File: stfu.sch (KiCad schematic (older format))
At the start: 91 parts, among them K1 FTDI, K2 ISP, K3 I2C, K4 SERVO, K5 V_SEL, P1 CONN_1, P2 CONN_1, P3 HAND_HI, P4 HAND_LO, P5 HAND_HI, P6 HAND_LO, Q1 PNP, SW1 RST, SW2 RST, SW3 SW_MODE, SW4 SW_INC, SW5 SW_DEC, SW6 SW_ENT, U1 ATMEGA328-P, U2 HEF4051B, U3 ULN2803, U4 7809, U5 7805, X1 16MHz

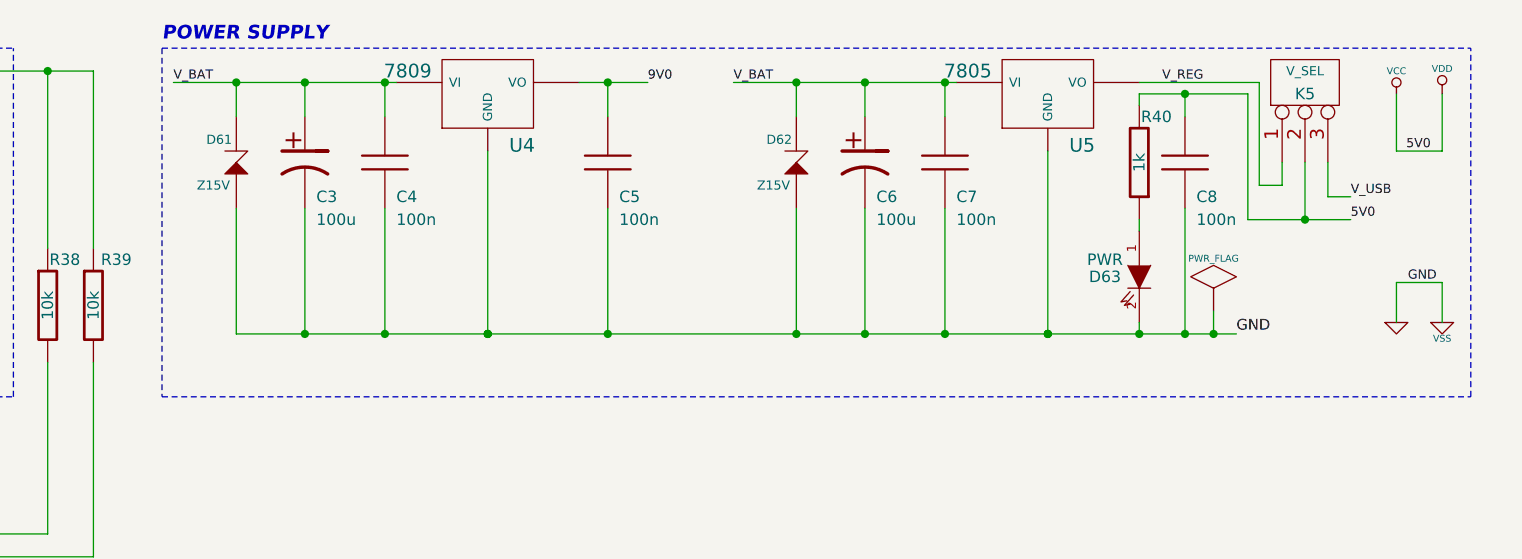
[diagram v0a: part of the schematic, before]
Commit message: preliminary board layout
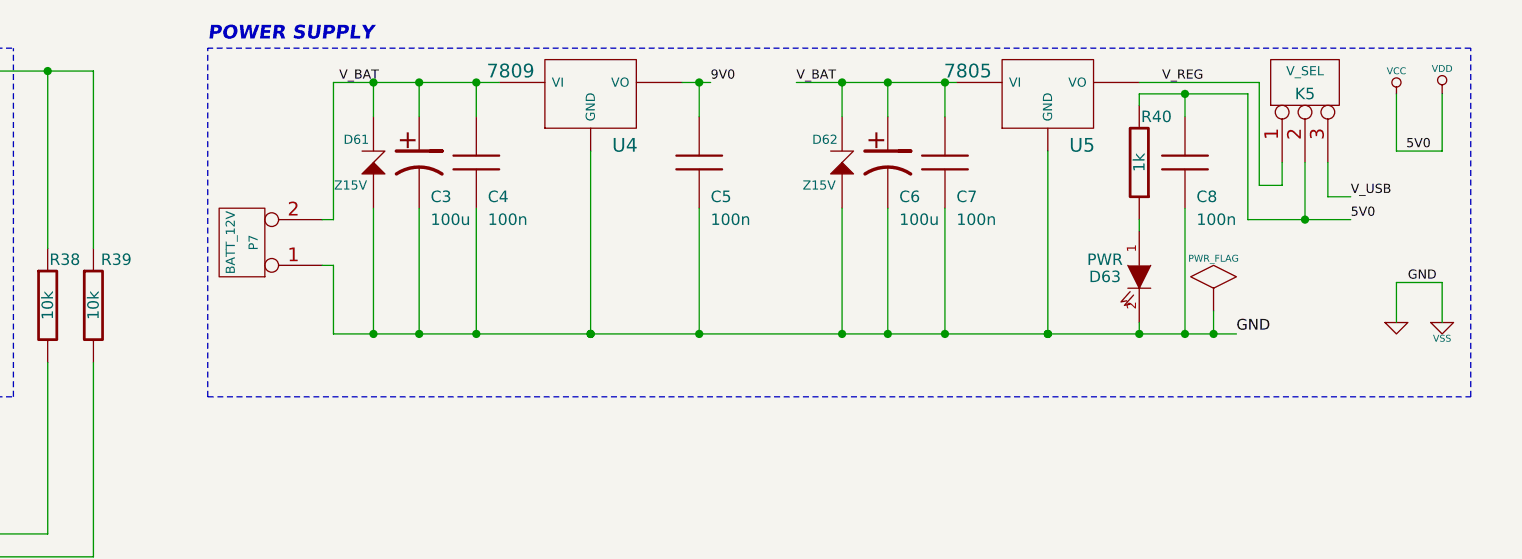
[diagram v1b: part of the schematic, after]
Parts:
- added P7: BATT_12V, symbol CONN_2
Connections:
- net GND: now also P7.1 (P1)
- net V_BAT: now also P7.2 (PM)
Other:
- moved on the sheet: C3, C4, C5, C6, D61, D62, U4
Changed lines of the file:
@@
-EESchema Schematic File Version 2  date 7/5/2012 5:41:43 PM
+EESchema Schematic File Version 2  date Monday 09 July 2012 12:59:22 AM IST
 LIBS:stfu
 LIBS:power
@@
 Sheet 1 2
 Title "STFU - a warning for incessant Noise polluters"
-Date "5 jul 2012"
+Date "8 jul 2012"
 Rev "A"
 Comp "anool.m@gmail.com"
@@
 $EndDescr
 Wire Notes Line
+	5600 2150 11125 2150
+Wire Notes Line
+	5600 2150 5600 625
+Wire Wire Line
+	6150 1375 6150 775
+Wire Wire Line
+	6150 1375 6100 1375
+Wire Notes Line
 	6950 3050 6950 4900
 Wire Notes Line
@@
 Wire Wire Line
 	6750 7325 4750 7325
-Connection ~ 8175 1875
-Wire Wire Line
-	8175 1875 8175 1325
+Connection ~ 8375 1875
+Wire Wire Line
+	8375 1875 8375 1325
 Wire Notes Line
 	3500 625  4750 625
@@
 Wire Notes Line
 	4750 2150 4750 625
-Wire Notes Line
-	5400 625  5400 2150
 Wire Wire Line
 	4900 5025 4750 5025
 Wire Wire Line
 	4750 5025 4750 5075
-Connection ~ 7350 775
-Wire Wire Line
-	7350 925  7350 775
-Connection ~ 5725 775
-Wire Wire Line
-	5725 925  5725 775
-Connection ~ 6825 1875
-Connection ~ 6375 775
-Connection ~ 6375 1875
-Wire Wire Line
-	6375 1875 6375 1325
-Connection ~ 6825 1875
-Wire Wire Line
-	6025 1325 6025 1875
-Wire Wire Line
-	6025 775  6025 925
-Wire Wire Line
-	6825 1875 6825 1075
-Wire Wire Line
-	6375 775  6375 925
-Connection ~ 6025 775
-Wire Wire Line
-	6425 775  5450 775
-Wire Wire Line
-	5725 1325 5725 1875
-Connection ~ 6025 1875
+Connection ~ 7750 775
+Wire Wire Line
+	7750 925  7750 775
+Connection ~ 6325 775
+Wire Wire Line
+	6325 775  6325 925
+Connection ~ 7275 1875
+Connection ~ 6775 775
+Connection ~ 6775 1875
+Wire Wire Line
+	6775 1875 6775 1325
+Connection ~ 7275 1875
+Wire Wire Line
+	6525 1875 6525 1325
+Wire Wire Line
+	6525 775  6525 925
+Wire Wire Line
+	7275 1875 7275 1075
+Wire Wire Line
+	6775 925  6775 775
+Connection ~ 6525 775
+Wire Wire Line
+	6150 775  6875 775
+Wire Wire Line
+	6325 1325 6325 1875
+Connection ~ 6525 1875
 Wire Wire Line
 	6750 4150 7525 4150
@@
 Wire Wire Line
 	650  2150 600  2150
-Connection ~ 8475 1875
-Wire Wire Line
-	5725 1875 10100 1875
+Connection ~ 8575 1875
 Connection ~ 10875 6125
 Wire Wire Line
@@
 	1950 7125 2150 7125
 Wire Wire Line
-	8875 775  7900 775
-Connection ~ 8475 775
+	8875 775  8175 775
+Connection ~ 8575 775
 Connection ~ 9875 825
 Wire Wire Line
 	9875 925  9875 825
 Wire Wire Line
-	8825 925  8825 775
+	8825 775  8825 925
 Wire Wire Line
 	9675 1875 9675 1825
@@
 	9275 1875 9275 1075
 Wire Wire Line
-	8475 775  8475 925
+	8575 775  8575 925
 Connection ~ 9675 1875
 Wire Wire Line
-	8475 1875 8475 1325
+	8575 1875 8575 1325
 Connection ~ 9275 1875
 Wire Wire Line
@@
 Connection ~ 9875 1875
 Wire Wire Line
-	10000 1775 10000 1875
+	10000 1875 10000 1775
 Connection ~ 10000 1875
 Wire Wire Line
-	8175 775  8175 925
-Connection ~ 8175 775
+	8375 925  8375 775
+Connection ~ 8375 775
 Wire Wire Line
 	1250 2150 1250 2650
@@
 	7050 4050 6750 4050
 Wire Wire Line
-	7525 775  7225 775
-Wire Wire Line
-	7350 1875 7350 1325
-Connection ~ 7350 1875
-Wire Notes Line
-	5400 625  11125 625
-Wire Notes Line
-	5400 2150 11125 2150
+	7800 775  7675 775
+Wire Wire Line
+	7750 1875 7750 1325
+Connection ~ 7750 1875
 Wire Notes Line
 	11125 2150 11125 625
@@
 Wire Notes Line
 	11125 4900 6950 4900
+Wire Wire Line
+	6100 1575 6150 1575
+Wire Wire Line
+	6150 1575 6150 1875
+Wire Wire Line
+	6150 1875 10100 1875
+Connection ~ 6325 1875
+Wire Notes Line
+	11125 625  5600 625
+$Comp
+L CONN_2 P7
+U 1 1 4FF99A4C
+P 5750 1475
+F 0 "P7" V 5700 1475 40  0000 C CNN
+F 1 "BATT_12V" V 5800 1475 40  0000 C CNN
+	1    5750 1475
+	-1   0    0    1
+$EndComp
 Text Label 9675 3350 0    40   ~ 0
 9V0_LH
@@
 L C C5
 U 1 1 4FF2E982
-P 7350 1125
-F 0 "C5" H 7400 975 50  0000 L CNN
-F 1 "100n" H 7400 875 50  0000 L CNN
-F 2 "C2" H 7350 1125 60  0001 C CNN
-	1    7350 1125
-	1    0    0    -1
-$EndComp
-Text Label 7525 775  0    40   ~ 0
+P 7750 1125
+F 0 "C5" H 7800 975 50  0000 L CNN
+F 1 "100n" H 7800 875 50  0000 L CNN
+F 2 "C2" H 7750 1125 60  0001 C CNN
+	1    7750 1125
+	1    0    0    -1
+$EndComp
+Text Label 7800 775  0    40   ~ 0
 9V0
 $Comp
 L DIODE_ZENER D61
 U 1 1 4FF2E927
-P 5725 1125
-F 0 "D61" V 5825 1200 40  0000 C CNN
-F 1 "Z15V" V 5625 1225 40  0000 C CNN
-F 2 "DO-35_Vert" H 5725 1125 60  0001 C CNN
-	1    5725 1125
+P 6325 1125
+F 0 "D61" V 6425 1200 40  0000 C CNN
+F 1 "Z15V" V 6225 1225 40  0000 C CNN
+F 2 "DO-35_Vert" H 6325 1125 60  0001 C CNN
+	1    6325 1125
 	0    -1   -1   0
 $EndComp
@@
 L CP1 C3
 U 1 1 4FF2E926
-P 6025 1125
-F 0 "C3" H 6075 975 50  0000 L CNN
-F 1 "100u" H 6075 875 50  0000 L CNN
-F 2 "CP_5x11mm" H 6025 1125 60  0001 C CNN
-	1    6025 1125
+P 6525 1125
+F 0 "C3" H 6575 975 50  0000 L CNN
+F 1 "100u" H 6575 875 50  0000 L CNN
+F 2 "CP_5x11mm" H 6525 1125 60  0001 C CNN
+	1    6525 1125
 	1    0    0    -1
 $EndComp
@@
 L C C4
 U 1 1 4FF2E925
-P 6375 1125
-F 0 "C4" H 6425 975 50  0000 L CNN
-F 1 "100n" H 6425 875 50  0000 L CNN
-F 2 "C2" H 6375 1125 60  0001 C CNN
-	1    6375 1125
-	1    0    0    -1
-$EndComp
-Text Label 5450 775  0    40   ~ 0
+P 6775 1125
+F 0 "C4" H 6825 975 50  0000 L CNN
+F 1 "100n" H 6825 875 50  0000 L CNN
+F 2 "C2" H 6775 1125 60  0001 C CNN
+	1    6775 1125
+	1    0    0    -1
+$EndComp
+Text Label 6175 775  0    40   ~ 0
 V_BAT
 $Comp
 L 7805 U4
 U 1 1 4FF2E924
-P 6825 825
-F 0 "U4" H 6975 600 60  0000 C CNN
-F 1 "7809" H 6475 925 60  0000 C CNN
-F 2 "TO-220_Vertical" H 6825 825 60  0001 C CNN
-	1    6825 825
+P 7275 825
+F 0 "U4" H 7425 600 60  0000 C CNN
+F 1 "7809" H 6925 925 60  0000 C CNN
+F 2 "TO-220_Vertical" H 7275 825 60  0001 C CNN
+	1    7275 825
 	1    0    0    -1
 $EndComp
@@
 $EndComp
 $Comp
-L GND #PWR01
+L GND #PWR1
 U 1 1 4FF29B8E
 P 1050 3650
-F 0 "#PWR01" H 1050 3650 30  0001 C CNN
+F 0 "#PWR1" H 1050 3650 30  0001 C CNN
 F 1 "GND" H 1050 3580 30  0001 C CNN
 	1    1050 3650
@@
 $EndComp
 $Comp
-L GND #PWR02
+L GND #PWR2
 U 1 1 4FF29B8D
 P 1250 2650
-F 0 "#PWR02" H 1250 2650 30  0001 C CNN
+F 0 "#PWR2" H 1250 2650 30  0001 C CNN
 F 1 "GND" H 1250 2580 30  0001 C CNN
 	1    1250 2650
@@
 $EndComp
 $Comp
-L VCC #PWR03
+L VCC #PWR3
 U 1 1 4FF29B8C
 P 2350 1550
-F 0 "#PWR03" H 2350 1650 30  0001 C CNN
+F 0 "#PWR3" H 2350 1650 30  0001 C CNN
 F 1 "VCC" H 2350 1650 30  0000 C CNN
 	1    2350 1550
@@
 $EndComp
 $Comp
-L GND #PWR04
+L GND #PWR4
 U 1 1 4FF29B8B
 P 2350 5025
-F 0 "#PWR04" H 2350 5025 30  0001 C CNN
+F 0 "#PWR4" H 2350 5025 30  0001 C CNN
 F 1 "GND" H 2350 4955 30  0001 C CNN
 	1    2350 5025
@@
 $EndComp
 $Comp
-L GND #PWR05
+L GND #PWR5
 U 1 1 4FF29B88
 P 2650 2100
-F 0 "#PWR05" H 2650 2100 30  0001 C CNN
+F 0 "#PWR5" H 2650 2100 30  0001 C CNN
 F 1 "GND" H 2650 2030 30  0001 C CNN
 	1    2650 2100
@@
 $EndComp
 $Comp
-L VCC #PWR06
+L VCC #PWR6
 U 1 1 4FF29B70
 P 10800 825
-F 0 "#PWR06" H 10800 925 30  0001 C CNN
+F 0 "#PWR6" H 10800 925 30  0001 C CNN
 F 1 "VCC" H 10800 925 30  0000 C CNN
 	1    10800 825
@@
 $EndComp
 $Comp
-L GND #PWR07
+L GND #PWR7
 U 1 1 4FF29B6F
 P 10800 1825
-F 0 "#PWR07" H 10800 1825 30  0001 C CNN
+F 0 "#PWR7" H 10800 1825 30  0001 C CNN
 F 1 "GND" H 10800 1755 30  0001 C CNN
 	1    10800 1825
@@
 $EndComp
 $Comp
-L VDD #PWR08
+L VDD #PWR9
 U 1 1 4FF29B6D
 P 11000 825
-F 0 "#PWR08" H 11000 925 30  0001 C CNN
+F 0 "#PWR9" H 11000 925 30  0001 C CNN
 F 1 "VDD" H 11000 935 30  0000 C CNN
 	1    11000 825
@@
 RES
 $Comp
-L VSS #PWR09
+L VSS #PWR10
 U 1 1 4FF29B6B
 P 11000 1825
-F 0 "#PWR09" H 11000 1825 30  0001 C CNN
+F 0 "#PWR10" H 11000 1825 30  0001 C CNN
 F 1 "VSS" H 11000 1755 30  0000 C CNN
 	1    11000 1825
@@
 ISP
 $Comp
-L PWR_FLAG #FLG010
+L PWR_FLAG #FLG1
 U 1 1 4FF29B6A
 P 10000 1775
-F 0 "#FLG010" H 10000 2045 30  0001 C CNN
+F 0 "#FLG1" H 10000 2045 30  0001 C CNN
 F 1 "PWR_FLAG" H 10000 2005 30  0000 C CNN
 	1    10000 1775
@@
 	1    0    0    -1
 $EndComp
-Text Label 7900 775  0    40   ~ 0
+Text Label 8175 775  0    40   ~ 0
 V_BAT
 Text Label 10600 1375 0    40   ~ 0
@@
 L CP1 C6
 U 1 1 4FF29B62
-P 8475 1125
-F 0 "C6" H 8525 975 50  0000 L CNN
-F 1 "100u" H 8525 875 50  0000 L CNN
-F 2 "CP_5x11mm" H 8475 1125 60  0001 C CNN
-	1    8475 1125
-	1    0    0    -1
-$EndComp
-Text Notes 5400 600  0    60   Italic 12
+P 8575 1125
+F 0 "C6" H 8625 975 50  0000 L CNN
+F 1 "100u" H 8625 875 50  0000 L CNN
+F 2 "CP_5x11mm" H 8575 1125 60  0001 C CNN
+	1    8575 1125
+	1    0    0    -1
+$EndComp
+Text Notes 5600 600  0    60   Italic 12
 POWER SUPPLY
 Text Label 3500 2550 0    40   ~ 0
@@
 MOUNTING HOLES
 $Comp
-L GND #PWR011
+L GND #PWR8
 U 1 1 4FF29B54
 P 10875 6225
-F 0 "#PWR011" H 10875 6225 30  0001 C CNN
+F 0 "#PWR8" H 10875 6225 30  0001 C CNN
 F 1 "GND" H 10875 6155 30  0001 C CNN
 	1    10875 6225
@@
 L DIODE_ZENER D62
 U 1 1 4FF29B4B
-P 8175 1125
-F 0 "D62" V 8275 1200 40  0000 C CNN
-F 1 "Z15V" V 8075 1225 40  0000 C CNN
-F 2 "DO-35_Vert" H 8175 1125 60  0001 C CNN
-	1    8175 1125
+P 8375 1125
+F 0 "D62" V 8475 1200 40  0000 C CNN
+F 1 "Z15V" V 8275 1225 40  0000 C CNN
+F 2 "DO-35_Vert" H 8375 1125 60  0001 C CNN
+	1    8375 1125
 	0    -1   -1   0
 $EndComp
